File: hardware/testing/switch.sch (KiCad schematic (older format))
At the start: 32 parts

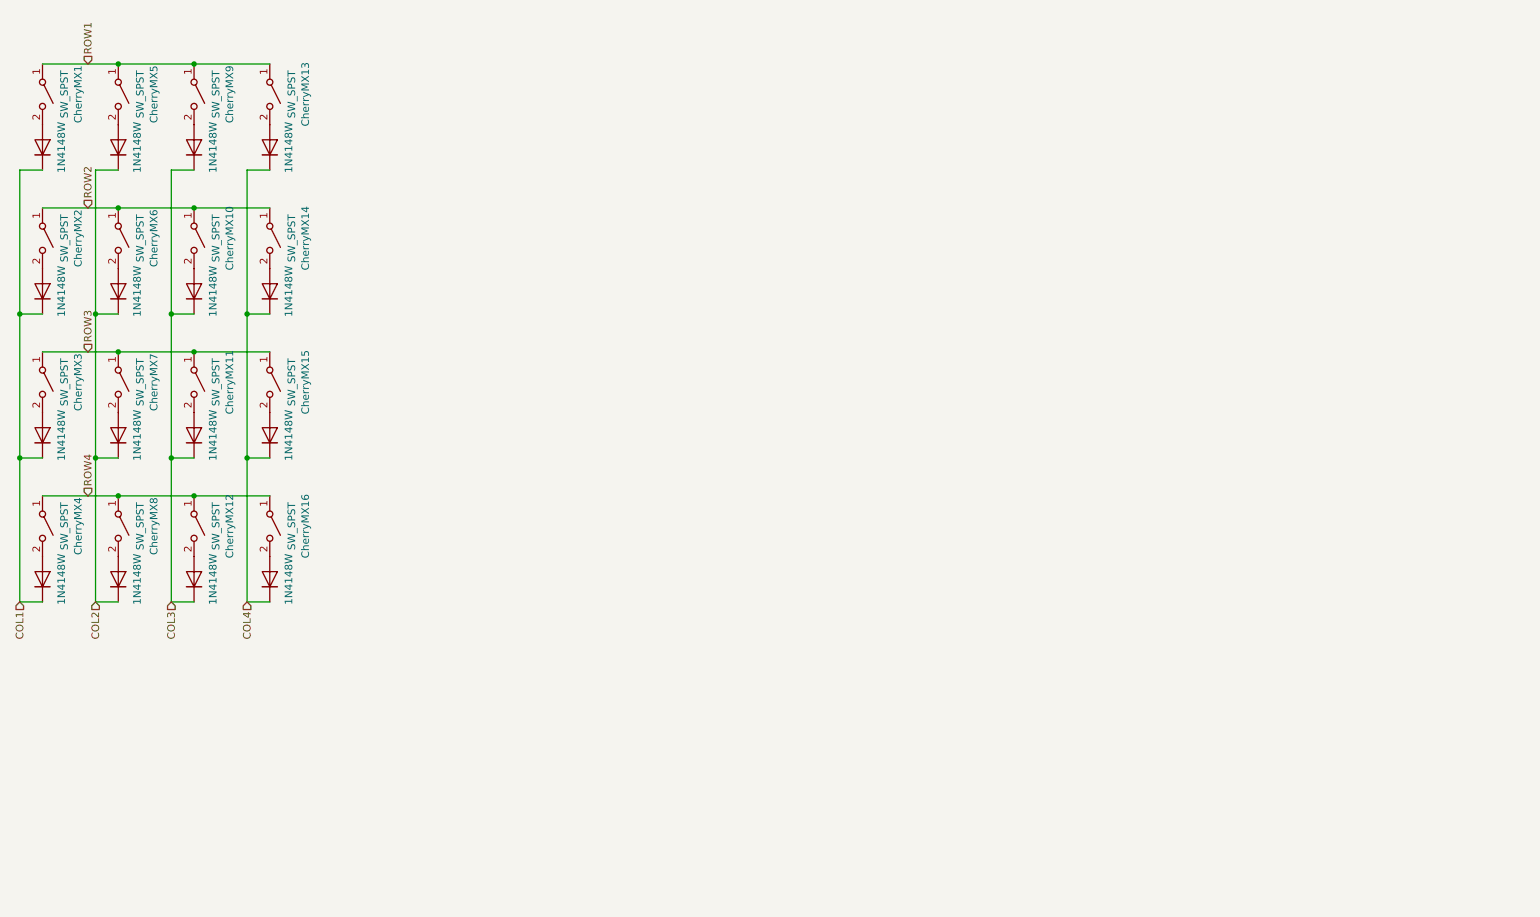
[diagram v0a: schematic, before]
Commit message: starting the testing PCB
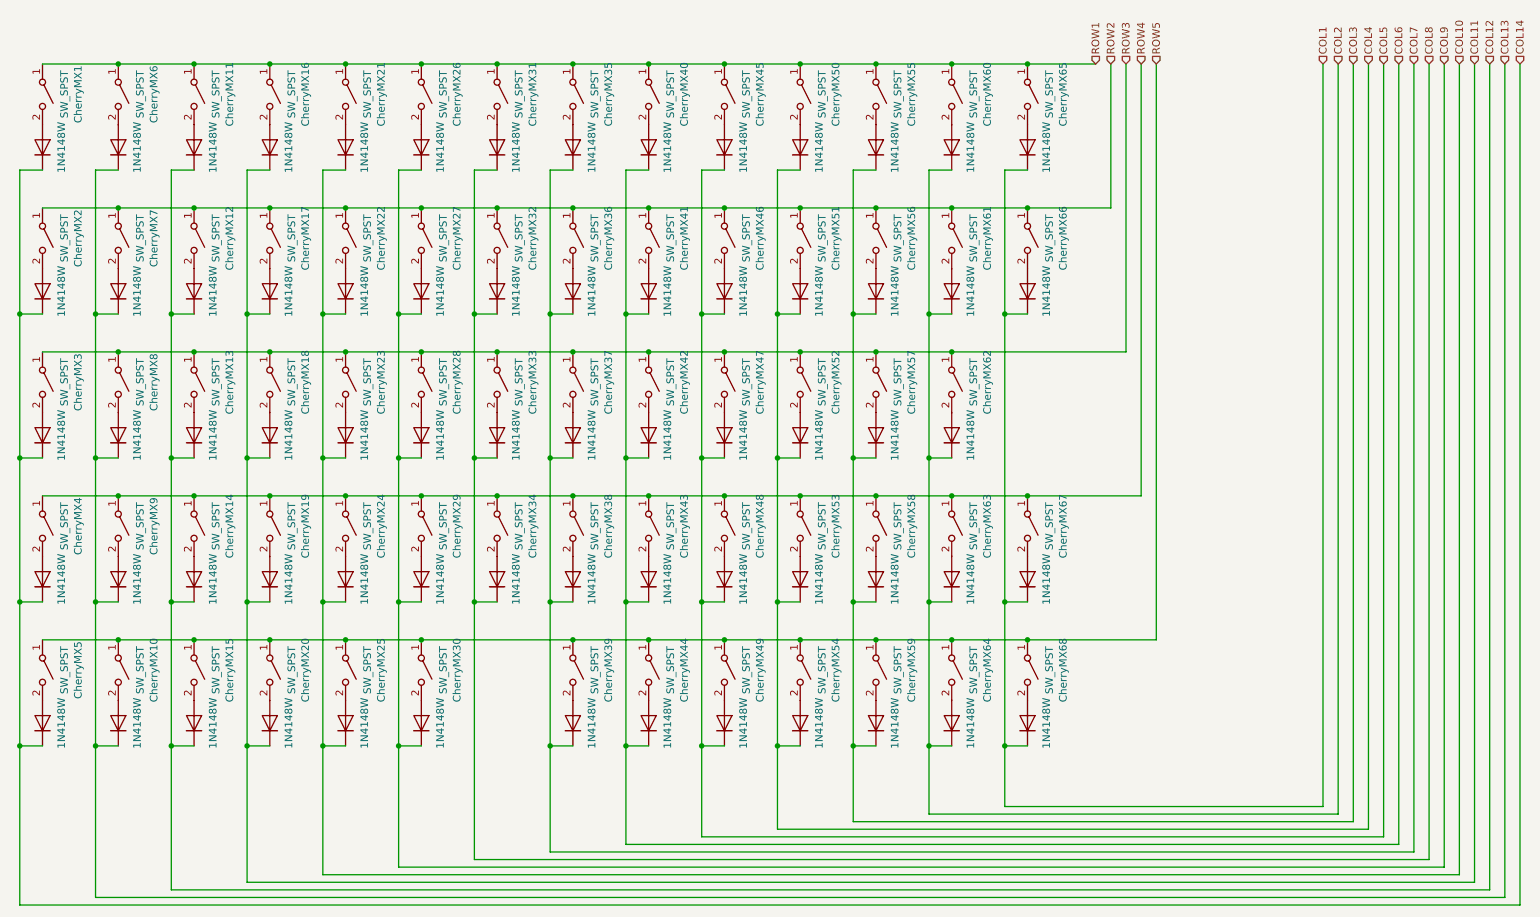
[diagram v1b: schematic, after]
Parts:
- added CherryMX10, CherryMX15, CherryMX20, CherryMX21, CherryMX22, CherryMX23, CherryMX24, CherryMX25, CherryMX26, CherryMX27, CherryMX28, CherryMX29, CherryMX30, CherryMX31, CherryMX32, CherryMX33, CherryMX34, CherryMX35, CherryMX36, CherryMX37, CherryMX38, CherryMX39, CherryMX40, CherryMX41, CherryMX42, CherryMX43, CherryMX44, CherryMX45, CherryMX46, CherryMX47, CherryMX48, CherryMX49, CherryMX5, CherryMX50, CherryMX51, CherryMX52, CherryMX53, CherryMX54, CherryMX55, CherryMX56, CherryMX57, CherryMX58, CherryMX59, CherryMX60, CherryMX61, CherryMX62, CherryMX63, CherryMX64, CherryMX65, CherryMX66, CherryMX67, CherryMX68: SW_SPST, TestPoint:TestPoint_2Pads_Pitch2.54mm_Drill0.8mm, symbol Switch:SW_SPST
- added D10, D15, D20, D21, D22, D23, D24, D25, D26, D27, D28, D29, D30, D31, D32, D33, D34, D35, D36, D37, D38, D39, D40, D41, D42, D43, D44, D45, D46, D47, D48, D49, D5, D50, D51, D52, D53, D54, D55, D56, D57, D58, D59, D60, D61, D62, D63, D64, D65, D66, D67, D68: 1N4148W, Diode_SMD:D_SOD-523, symbol Diode:1N4148W
- CherryMX1, CherryMX2, CherryMX3, CherryMX4: footprint Button_Switch_Keyboard:SW_Cherry_MX_1.00u_Plate -> TestPoint:TestPoint_2Pads_Pitch2.54mm_Drill0.8mm; Footprint (none) -> keyswitches:Kailh_socket_MX_optional_reversible
- CherryMX11: renamed from CherryMX9; footprint Button_Switch_Keyboard:SW_Cherry_MX_1.00u_Plate -> TestPoint:TestPoint_2Pads_Pitch2.54mm_Drill0.8mm; Footprint (none) -> keyswitches:Kailh_socket_MX_optional_reversible
- CherryMX12: renamed from CherryMX10; footprint Button_Switch_Keyboard:SW_Cherry_MX_1.00u_Plate -> TestPoint:TestPoint_2Pads_Pitch2.54mm_Drill0.8mm; Footprint (none) -> keyswitches:Kailh_socket_MX_optional_reversible
- CherryMX13: renamed from CherryMX11; footprint Button_Switch_Keyboard:SW_Cherry_MX_1.00u_Plate -> TestPoint:TestPoint_2Pads_Pitch2.54mm_Drill0.8mm; Footprint (none) -> keyswitches:Kailh_socket_MX_optional_reversible
- CherryMX14: renamed from CherryMX12; footprint Button_Switch_Keyboard:SW_Cherry_MX_1.00u_Plate -> TestPoint:TestPoint_2Pads_Pitch2.54mm_Drill0.8mm; Footprint (none) -> keyswitches:Kailh_socket_MX_optional_reversible
- CherryMX16: renamed from CherryMX13; footprint Button_Switch_Keyboard:SW_Cherry_MX_1.00u_Plate -> TestPoint:TestPoint_2Pads_Pitch2.54mm_Drill0.8mm; Footprint (none) -> keyswitches:Kailh_socket_MX_optional_reversible
- CherryMX17: renamed from CherryMX14; footprint Button_Switch_Keyboard:SW_Cherry_MX_1.00u_Plate -> TestPoint:TestPoint_2Pads_Pitch2.54mm_Drill0.8mm; Footprint (none) -> keyswitches:Kailh_socket_MX_optional_reversible
- CherryMX18: renamed from CherryMX15; footprint Button_Switch_Keyboard:SW_Cherry_MX_1.00u_Plate -> TestPoint:TestPoint_2Pads_Pitch2.54mm_Drill0.8mm; Footprint (none) -> keyswitches:Kailh_socket_MX_optional_reversible
- CherryMX19: renamed from CherryMX16; footprint Button_Switch_Keyboard:SW_Cherry_MX_1.00u_Plate -> TestPoint:TestPoint_2Pads_Pitch2.54mm_Drill0.8mm; Footprint (none) -> keyswitches:Kailh_socket_MX_optional_reversible
- CherryMX6: renamed from CherryMX5; footprint Button_Switch_Keyboard:SW_Cherry_MX_1.00u_Plate -> TestPoint:TestPoint_2Pads_Pitch2.54mm_Drill0.8mm; Footprint (none) -> keyswitches:Kailh_socket_MX_optional_reversible
- CherryMX7: renamed from CherryMX6; footprint Button_Switch_Keyboard:SW_Cherry_MX_1.00u_Plate -> TestPoint:TestPoint_2Pads_Pitch2.54mm_Drill0.8mm; Footprint (none) -> keyswitches:Kailh_socket_MX_optional_reversible
- CherryMX8: renamed from CherryMX7; footprint Button_Switch_Keyboard:SW_Cherry_MX_1.00u_Plate -> TestPoint:TestPoint_2Pads_Pitch2.54mm_Drill0.8mm; Footprint (none) -> keyswitches:Kailh_socket_MX_optional_reversible
- CherryMX9: renamed from CherryMX8; footprint Button_Switch_Keyboard:SW_Cherry_MX_1.00u_Plate -> TestPoint:TestPoint_2Pads_Pitch2.54mm_Drill0.8mm; Footprint (none) -> keyswitches:Kailh_socket_MX_optional_reversible
- D1, D2, D3, D4: footprint Diode_SMD:D_SOD-123 -> Diode_SMD:D_SOD-523; Footprint (none) -> Diode_SMD:D_SOD-123
- D11: renamed from D9; footprint Diode_SMD:D_SOD-123 -> Diode_SMD:D_SOD-523; Footprint (none) -> Diode_SMD:D_SOD-123
- D12: renamed from D10; footprint Diode_SMD:D_SOD-123 -> Diode_SMD:D_SOD-523; Footprint (none) -> Diode_SMD:D_SOD-123
- D13: renamed from D11; footprint Diode_SMD:D_SOD-123 -> Diode_SMD:D_SOD-523; Footprint (none) -> Diode_SMD:D_SOD-123
- D14: renamed from D12; footprint Diode_SMD:D_SOD-123 -> Diode_SMD:D_SOD-523; Footprint (none) -> Diode_SMD:D_SOD-123
- D16: renamed from D13; footprint Diode_SMD:D_SOD-123 -> Diode_SMD:D_SOD-523; Footprint (none) -> Diode_SMD:D_SOD-123
- D17: renamed from D14; footprint Diode_SMD:D_SOD-123 -> Diode_SMD:D_SOD-523; Footprint (none) -> Diode_SMD:D_SOD-123
- D18: renamed from D15; footprint Diode_SMD:D_SOD-123 -> Diode_SMD:D_SOD-523; Footprint (none) -> Diode_SMD:D_SOD-123
- D19: renamed from D16; footprint Diode_SMD:D_SOD-123 -> Diode_SMD:D_SOD-523; Footprint (none) -> Diode_SMD:D_SOD-123
- D6: renamed from D5; footprint Diode_SMD:D_SOD-123 -> Diode_SMD:D_SOD-523; Footprint (none) -> Diode_SMD:D_SOD-123
- D7: renamed from D6; footprint Diode_SMD:D_SOD-123 -> Diode_SMD:D_SOD-523; Footprint (none) -> Diode_SMD:D_SOD-123
- D8: renamed from D7; footprint Diode_SMD:D_SOD-123 -> Diode_SMD:D_SOD-523; Footprint (none) -> Diode_SMD:D_SOD-123
- D9: renamed from D8; footprint Diode_SMD:D_SOD-123 -> Diode_SMD:D_SOD-523; Footprint (none) -> Diode_SMD:D_SOD-123
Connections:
- net COL1: now also D65.1 (K), D66.1 (K), D67.1 (K), D68.1 (K); no longer D1.1 (K), D2.1 (K), D3.1 (K), D4.1 (K)
- net COL2: now also D60.1 (K), D61.1 (K), D62.1 (K), D63.1 (K), D64.1 (K); no longer D6.1 (K), D7.1 (K), D8.1 (K), D9.1 (K)
- net COL3: now also D55.1 (K), D56.1 (K), D57.1 (K), D58.1 (K), D59.1 (K); no longer D11.1 (K), D12.1 (K), D13.1 (K), D14.1 (K)
- net COL4: now also D50.1 (K), D51.1 (K), D52.1 (K), D53.1 (K), D54.1 (K); no longer D16.1 (K), D17.1 (K), D18.1 (K), D19.1 (K)
- net ROW1: now also CherryMX21.1 (A), CherryMX26.1 (A), CherryMX31.1 (A), CherryMX35.1 (A), CherryMX40.1 (A), CherryMX45.1 (A), CherryMX50.1 (A), CherryMX55.1 (A), CherryMX60.1 (A), CherryMX65.1 (A)
- net ROW2: now also CherryMX22.1 (A), CherryMX27.1 (A), CherryMX32.1 (A), CherryMX36.1 (A), CherryMX41.1 (A), CherryMX46.1 (A), CherryMX51.1 (A), CherryMX56.1 (A), CherryMX61.1 (A), CherryMX66.1 (A)
- net ROW3: now also CherryMX23.1 (A), CherryMX28.1 (A), CherryMX33.1 (A), CherryMX37.1 (A), CherryMX42.1 (A), CherryMX47.1 (A), CherryMX52.1 (A), CherryMX57.1 (A), CherryMX62.1 (A)
- net ROW4: now also CherryMX24.1 (A), CherryMX29.1 (A), CherryMX34.1 (A), CherryMX38.1 (A), CherryMX43.1 (A), CherryMX48.1 (A), CherryMX53.1 (A), CherryMX58.1 (A), CherryMX63.1 (A), CherryMX67.1 (A)
- new net: CherryMX5.2 (B), D5.2 (A)
- new net: CherryMX10.2 (B), D10.2 (A)
- new net: CherryMX15.2 (B), D15.2 (A)
- new net: CherryMX20.2 (B), D20.2 (A)
- new net: CherryMX21.2 (B), D21.2 (A)
- new net: CherryMX22.2 (B), D22.2 (A)
- new net: CherryMX23.2 (B), D23.2 (A)
- new net: CherryMX24.2 (B), D24.2 (A)
- new net: CherryMX25.2 (B), D25.2 (A)
- new net: CherryMX26.2 (B), D26.2 (A)
- new net: CherryMX27.2 (B), D27.2 (A)
- new net: CherryMX28.2 (B), D28.2 (A)
- new net: CherryMX29.2 (B), D29.2 (A)
- new net: CherryMX30.2 (B), D30.2 (A)
- new net: CherryMX31.2 (B), D31.2 (A)
- new net: CherryMX32.2 (B), D32.2 (A)
- new net: CherryMX33.2 (B), D33.2 (A)
- new net: CherryMX34.2 (B), D34.2 (A)
- new net: CherryMX35.2 (B), D35.2 (A)
- new net: CherryMX36.2 (B), D36.2 (A)
- new net: CherryMX37.2 (B), D37.2 (A)
- new net: CherryMX38.2 (B), D38.2 (A)
- new net: CherryMX39.2 (B), D39.2 (A)
- new net: CherryMX40.2 (B), D40.2 (A)
- new net: CherryMX41.2 (B), D41.2 (A)
- new net: CherryMX42.2 (B), D42.2 (A)
- new net: CherryMX43.2 (B), D43.2 (A)
- new net: CherryMX44.2 (B), D44.2 (A)
- new net: CherryMX45.2 (B), D45.2 (A)
- new net: CherryMX46.2 (B), D46.2 (A)
- new net: CherryMX47.2 (B), D47.2 (A)
- new net: CherryMX48.2 (B), D48.2 (A)
- new net: CherryMX49.2 (B), D49.2 (A)
- new net: CherryMX50.2 (B), D50.2 (A)
- new net: CherryMX51.2 (B), D51.2 (A)
- new net: CherryMX52.2 (B), D52.2 (A)
- new net: CherryMX53.2 (B), D53.2 (A)
- new net: CherryMX54.2 (B), D54.2 (A)
- new net: CherryMX55.2 (B), D55.2 (A)
- new net: CherryMX56.2 (B), D56.2 (A)
- new net: CherryMX57.2 (B), D57.2 (A)
- new net: CherryMX58.2 (B), D58.2 (A)
- new net: CherryMX59.2 (B), D59.2 (A)
- new net: CherryMX60.2 (B), D60.2 (A)
- new net: CherryMX61.2 (B), D61.2 (A)
- new net: CherryMX62.2 (B), D62.2 (A)
- new net: CherryMX63.2 (B), D63.2 (A)
- new net: CherryMX64.2 (B), D64.2 (A)
- new net: CherryMX65.2 (B), D65.2 (A)
- new net: CherryMX66.2 (B), D66.2 (A)
- new net: CherryMX67.2 (B), D67.2 (A)
- new net: CherryMX68.2 (B), D68.2 (A)
- new net COL10: D21.1 (K), D22.1 (K), D23.1 (K), D24.1 (K), D25.1 (K)
- new net COL11: D16.1 (K), D17.1 (K), D18.1 (K), D19.1 (K), D20.1 (K)
- new net COL12: D11.1 (K), D12.1 (K), D13.1 (K), D14.1 (K), D15.1 (K)
- new net COL13: D10.1 (K), D6.1 (K), D7.1 (K), D8.1 (K), D9.1 (K)
- new net COL14: D1.1 (K), D2.1 (K), D3.1 (K), D4.1 (K), D5.1 (K)
- new net COL5: D45.1 (K), D46.1 (K), D47.1 (K), D48.1 (K), D49.1 (K)
- new net COL6: D40.1 (K), D41.1 (K), D42.1 (K), D43.1 (K), D44.1 (K)
- new net COL7: D35.1 (K), D36.1 (K), D37.1 (K), D38.1 (K), D39.1 (K)
- new net COL8: D31.1 (K), D32.1 (K), D33.1 (K), D34.1 (K)
- new net COL9: D26.1 (K), D27.1 (K), D28.1 (K), D29.1 (K), D30.1 (K)
- new net ROW5: CherryMX10.1 (A), CherryMX15.1 (A), CherryMX20.1 (A), CherryMX25.1 (A), CherryMX30.1 (A), CherryMX39.1 (A), CherryMX44.1 (A), CherryMX49.1 (A), CherryMX5.1 (A), CherryMX54.1 (A), CherryMX59.1 (A), CherryMX64.1 (A), CherryMX68.1 (A)
